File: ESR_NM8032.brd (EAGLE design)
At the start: 34.9 x 90.8 mm, 80 parts, among them J1 0

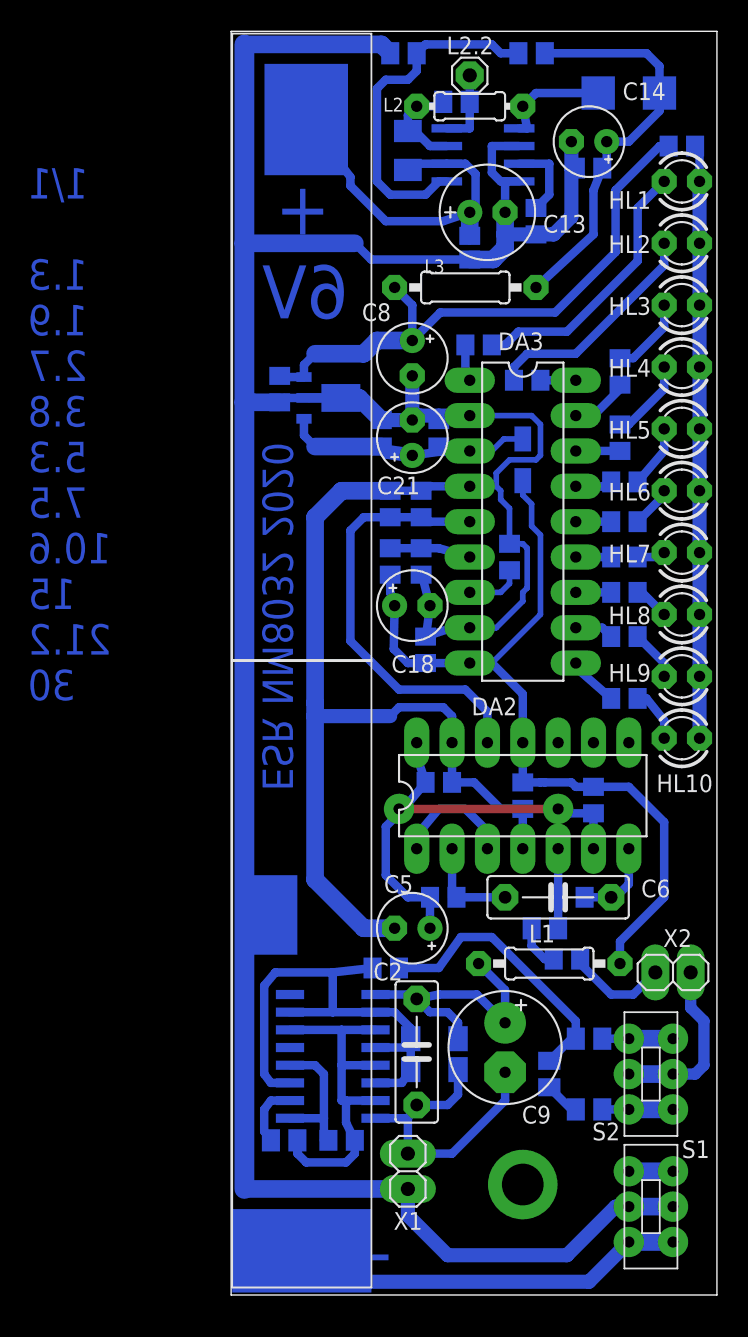
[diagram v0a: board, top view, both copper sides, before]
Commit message: .
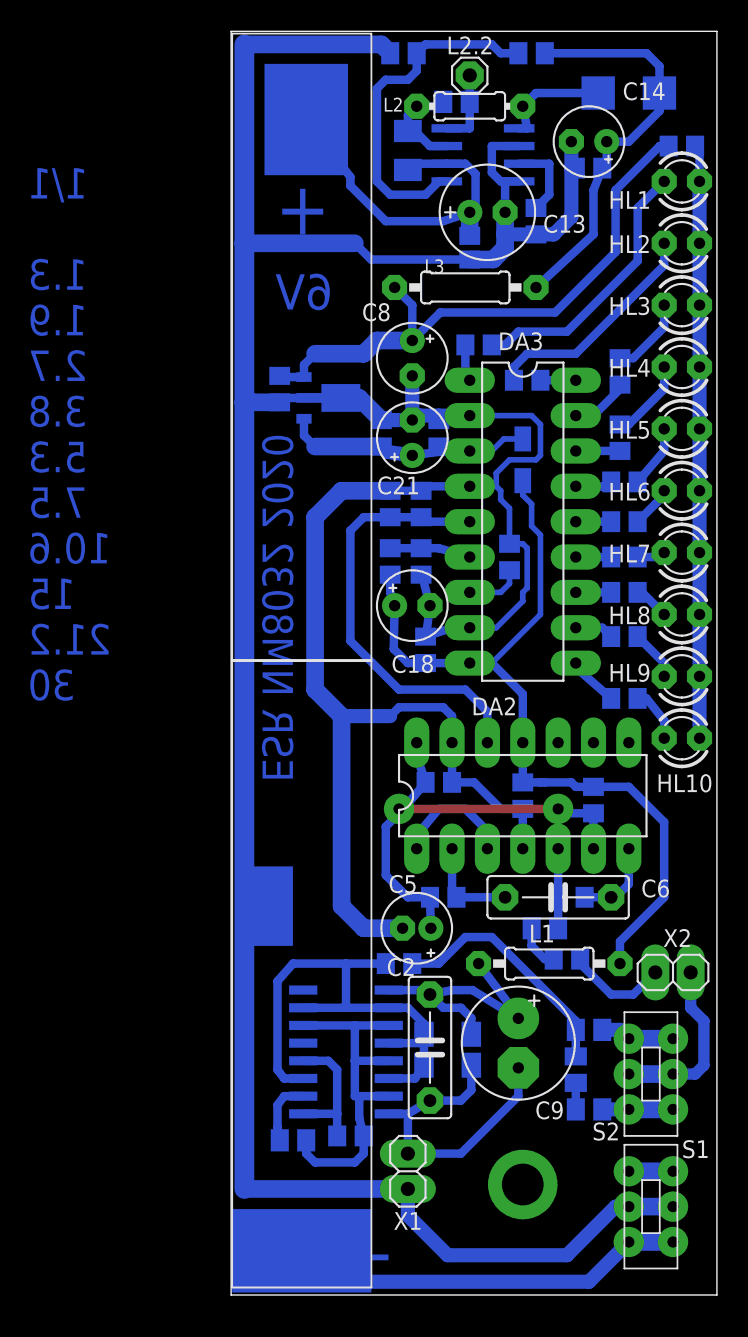
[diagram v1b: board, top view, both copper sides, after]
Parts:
- C5: device rcl:E2,5-5 -> rcl:E2-5
- moved R3 1.93 mm to (18.1, 41.3)
- moved C9 1.00 mm to (14.0, 43.2)
- moved VD2 1.00 mm to (8.89, 41.6)
- moved DD1 1.00 mm to (1.59, 42.5)
- moved C3 1.00 mm to (5.40, 48.9)
- moved VD1 1.00 mm to (8.89, 43.8)
- moved C2 1.00 mm to (7.62, 42.9)
- moved C1 0.71 mm to (1.91, 36.5)
- moved R1 0.63 mm to (-2.22, 36.2)
- moved R2 0.63 mm to (19.1, 44.1)
- moved C5 0.32 mm to (6.67, 51.4)
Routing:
- net N$26: track 20.2 -> 17.6 mm
- net GND: track 296.5 -> 294.8 mm
- net GNDS: track 21.7 -> 22.8 mm
- net N$17: track 2.57 -> 1.91 mm
